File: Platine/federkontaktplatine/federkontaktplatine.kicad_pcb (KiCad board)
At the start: 2 copper layers, 256 x 149 mm, 15 parts, among them J1 Conn_01x07

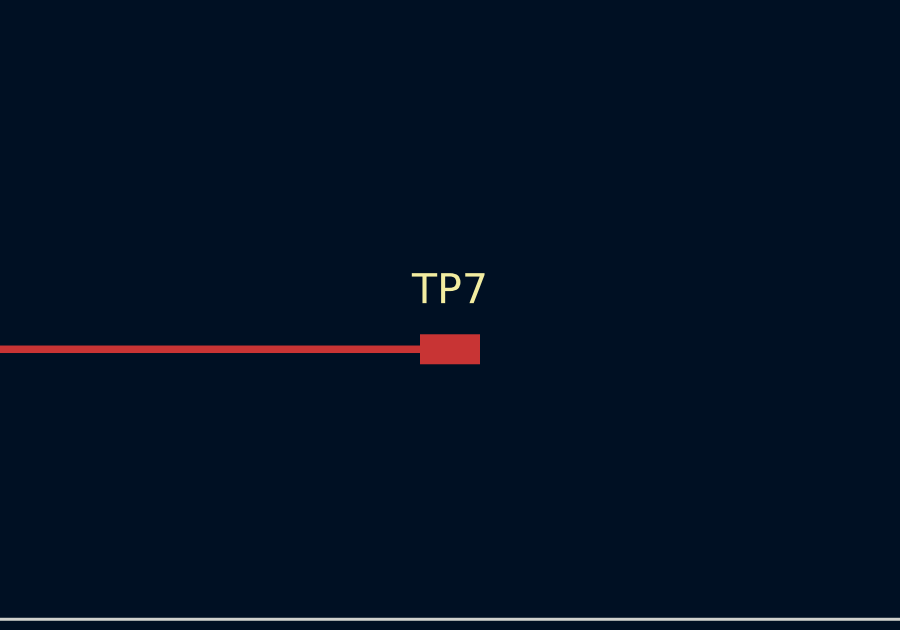
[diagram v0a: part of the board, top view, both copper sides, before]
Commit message: Platinen update
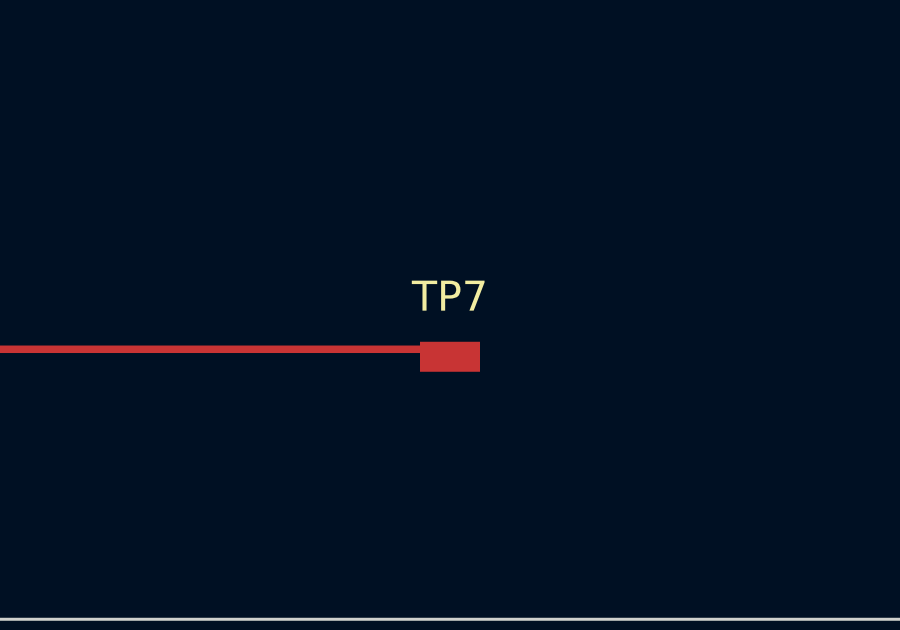
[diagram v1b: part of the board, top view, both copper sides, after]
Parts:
- moved TP7 0.25 mm to (191.0, 149.2)
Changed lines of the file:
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@@
   )
   (footprint "TestPoint:PAD_1x2mm" (layer "F.Cu")
-    (at 191 149)
+    (at 191 149.25)
     (property "Sheetfile" "federkontaktplatine.kicad_sch")
     (property "Sheetname" "")
